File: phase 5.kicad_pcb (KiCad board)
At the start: 2 copper layers, 48.9 x 44.1 mm, 14 parts, among them J4 USB_C_Receptacle_USB2.0, SW1 SW_PUSH, U1 ATMEGA32U2, Y1 Resonator

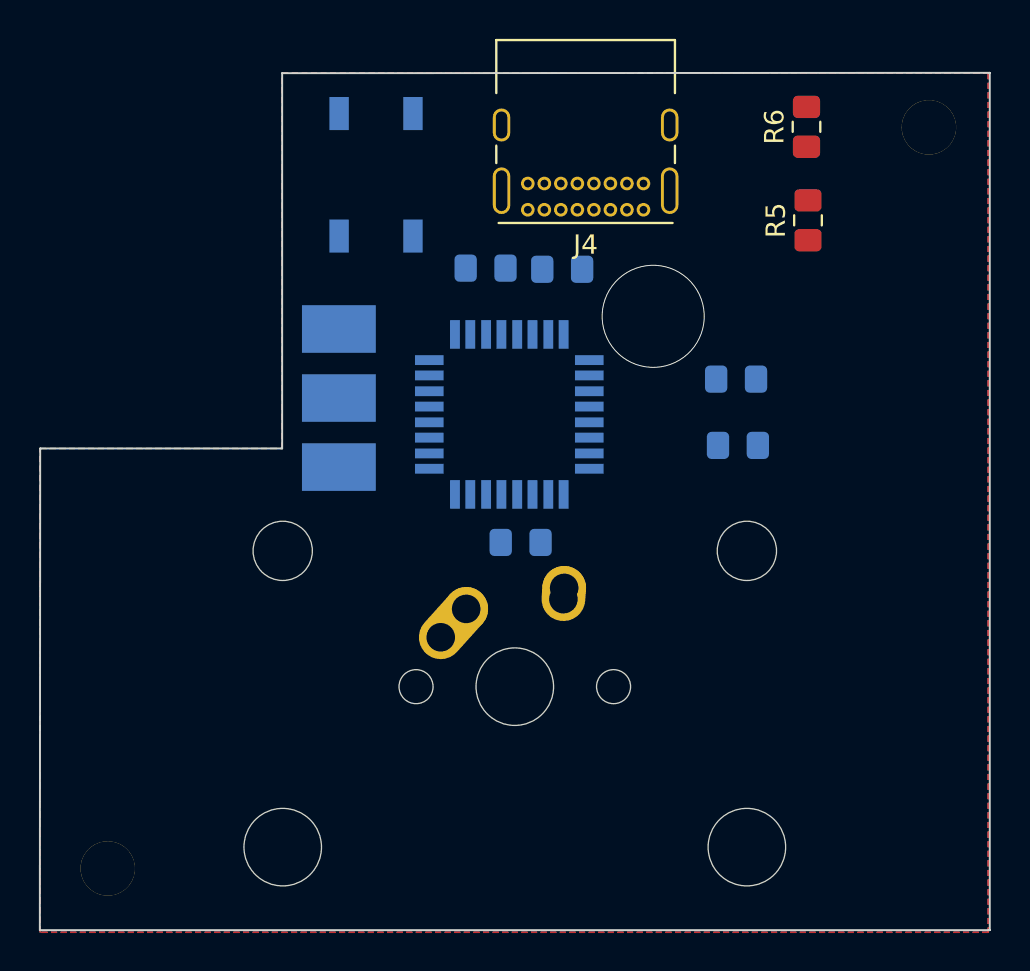
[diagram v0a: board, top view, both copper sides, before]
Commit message: Add files via upload
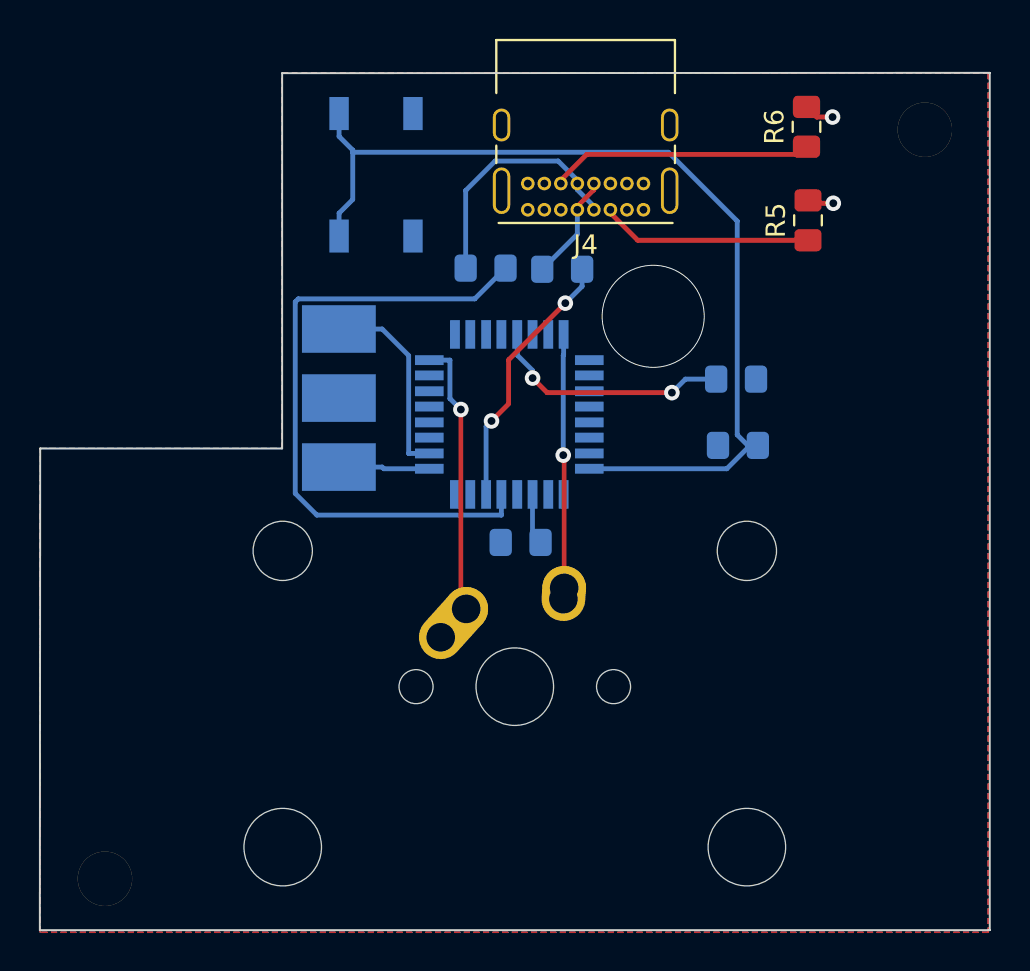
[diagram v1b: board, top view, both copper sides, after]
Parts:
- removed the HOLE_M2.6 at (20.5, 57.9)
- removed the HOLE_M2.6 at (62.7, 19.8)
- added HOLE_M2.6: VAL**, keyboard_parts:HOLE_M2.6, F.Cu at (62.5, 19.9)
- added HOLE_M2.6: VAL**, keyboard_parts:HOLE_M2.6, F.Cu at (20.3, 58.5)
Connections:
- K_BOTTOM_ENTER pad 1: col0 -> (no net)
- K_BOTTOM_ENTER pad 2: Net-(D_BOTTOM_ENTER-Pad2) -> (no net)
- U1 pad 16: row1 -> (no net)
- U1 pad 8: col0 -> (no net)
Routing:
- net Net-(R3-Pad2): track 0.00 -> 49.1 mm
- net Net-(R2-Pad2): track 0.00 -> 33.5 mm
- net (no net): track 0.00 -> 29.9 mm, vias 1 -> 2
- net Net-(R1-Pad2): track 0.00 -> 13.6 mm, vias 0 -> 2
- net Net-(J4-PadB5): track 0.00 -> 13.5 mm
- net Net-(J4-PadA6): track 0.00 -> 12.6 mm
- net Net-(R4-Pad1): track 0.00 -> 12.6 mm, vias 0 -> 2
- net Net-(J4-PadA5): track 0.00 -> 10.9 mm
- net Net-(U1-Pad2): track 0.00 -> 10.3 mm
- net Net-(J4-PadA7): track 0.00 -> 5.51 mm
- net Net-(U1-Pad1): track 0.00 -> 4.69 mm
- net GND: track 0.00 -> 2.92 mm, vias 0 -> 3
- net Net-(C1-Pad2): track 0.00 -> 2.64 mm
